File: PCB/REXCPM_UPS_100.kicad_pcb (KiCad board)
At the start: 2 copper layers, 51.3 x 18.3 mm, 14 parts, among them J1 Model_100_System_BUS, J2 SM04B, U1 742G02

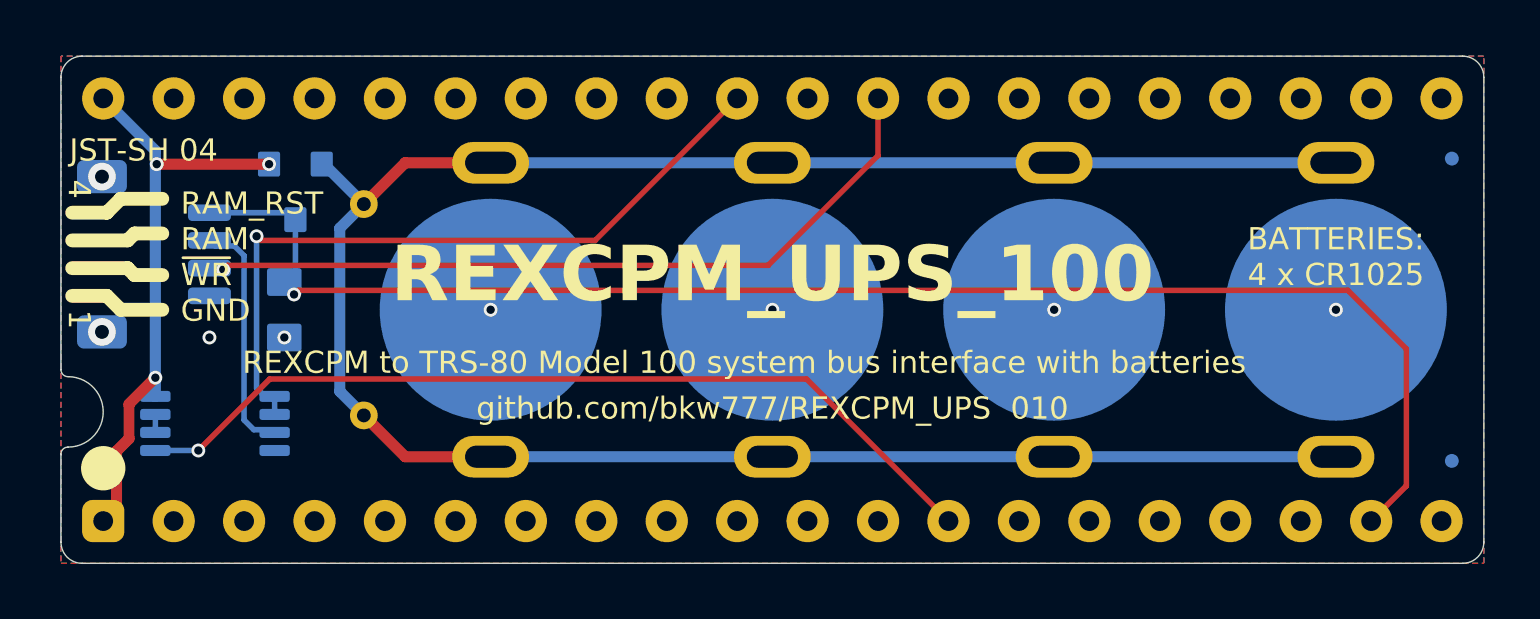
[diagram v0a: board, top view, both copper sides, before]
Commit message: batt footprint
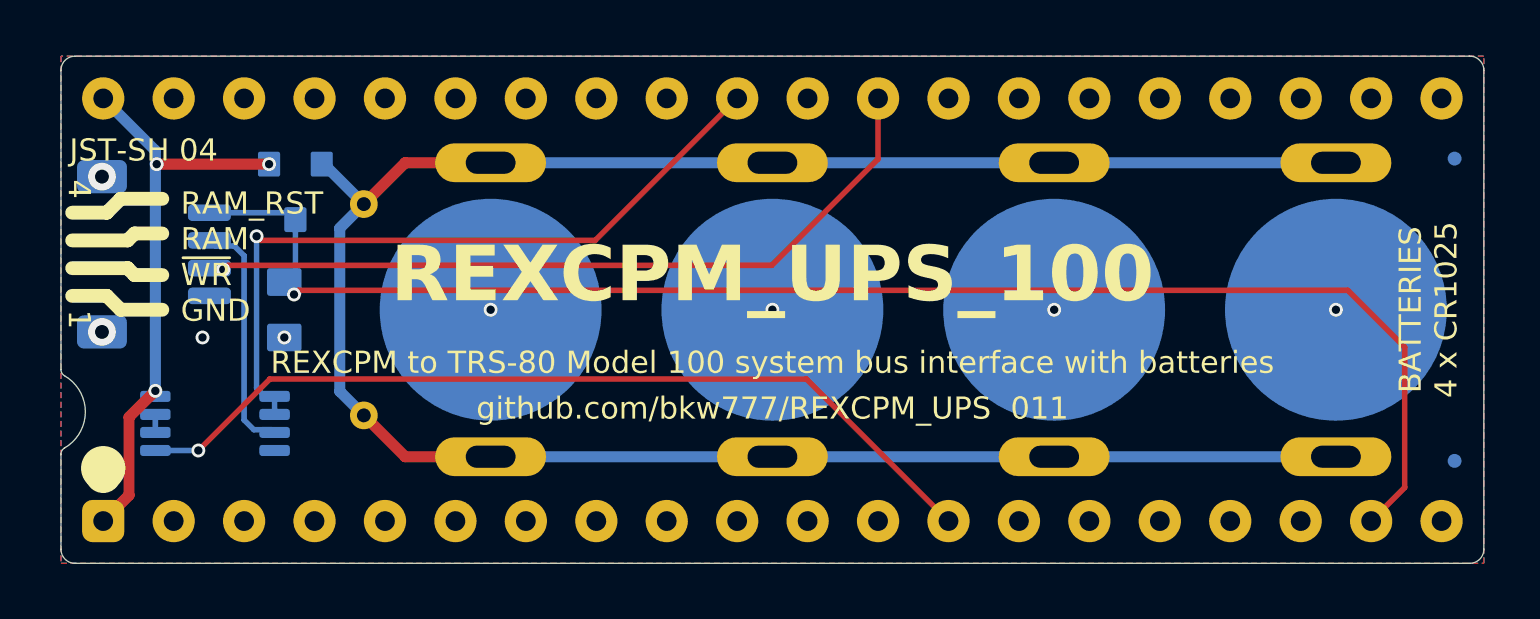
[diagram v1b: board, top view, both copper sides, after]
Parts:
- BT1, BT2, BT3, BT4: value Keystone_3031 -> BAT_3031
- J1: footprint 000_LOCAL:DIP-40_pins -> 000_LOCAL:DIP-40_PCB
- moved REF** 0.20 mm to (112.4, 110.2)
- moved REF** 0.10 mm to (161.1, 99.3)
- moved REF** 0.10 mm to (161.1, 110.2)
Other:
- outline, holes or cut-outs redrawn
- board text added: "BATTERIES 4 x CR1025"
- board text removed: "BATTERIES: 4 x CR1025"
